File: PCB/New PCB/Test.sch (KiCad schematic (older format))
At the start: 38 parts, among them P10 CONN_2, P11 CONN_2, P12 CONN_1, P13 CONN_1, P14 CONN_1, P15 CONN_1, P16 CONN_6, P2 PROG_H, P3 CONN_2, P6 CONN_2, P7 CONN_2, P8 CONN_2, P9 CONN_2, U1 DSPIC33EP512MC806

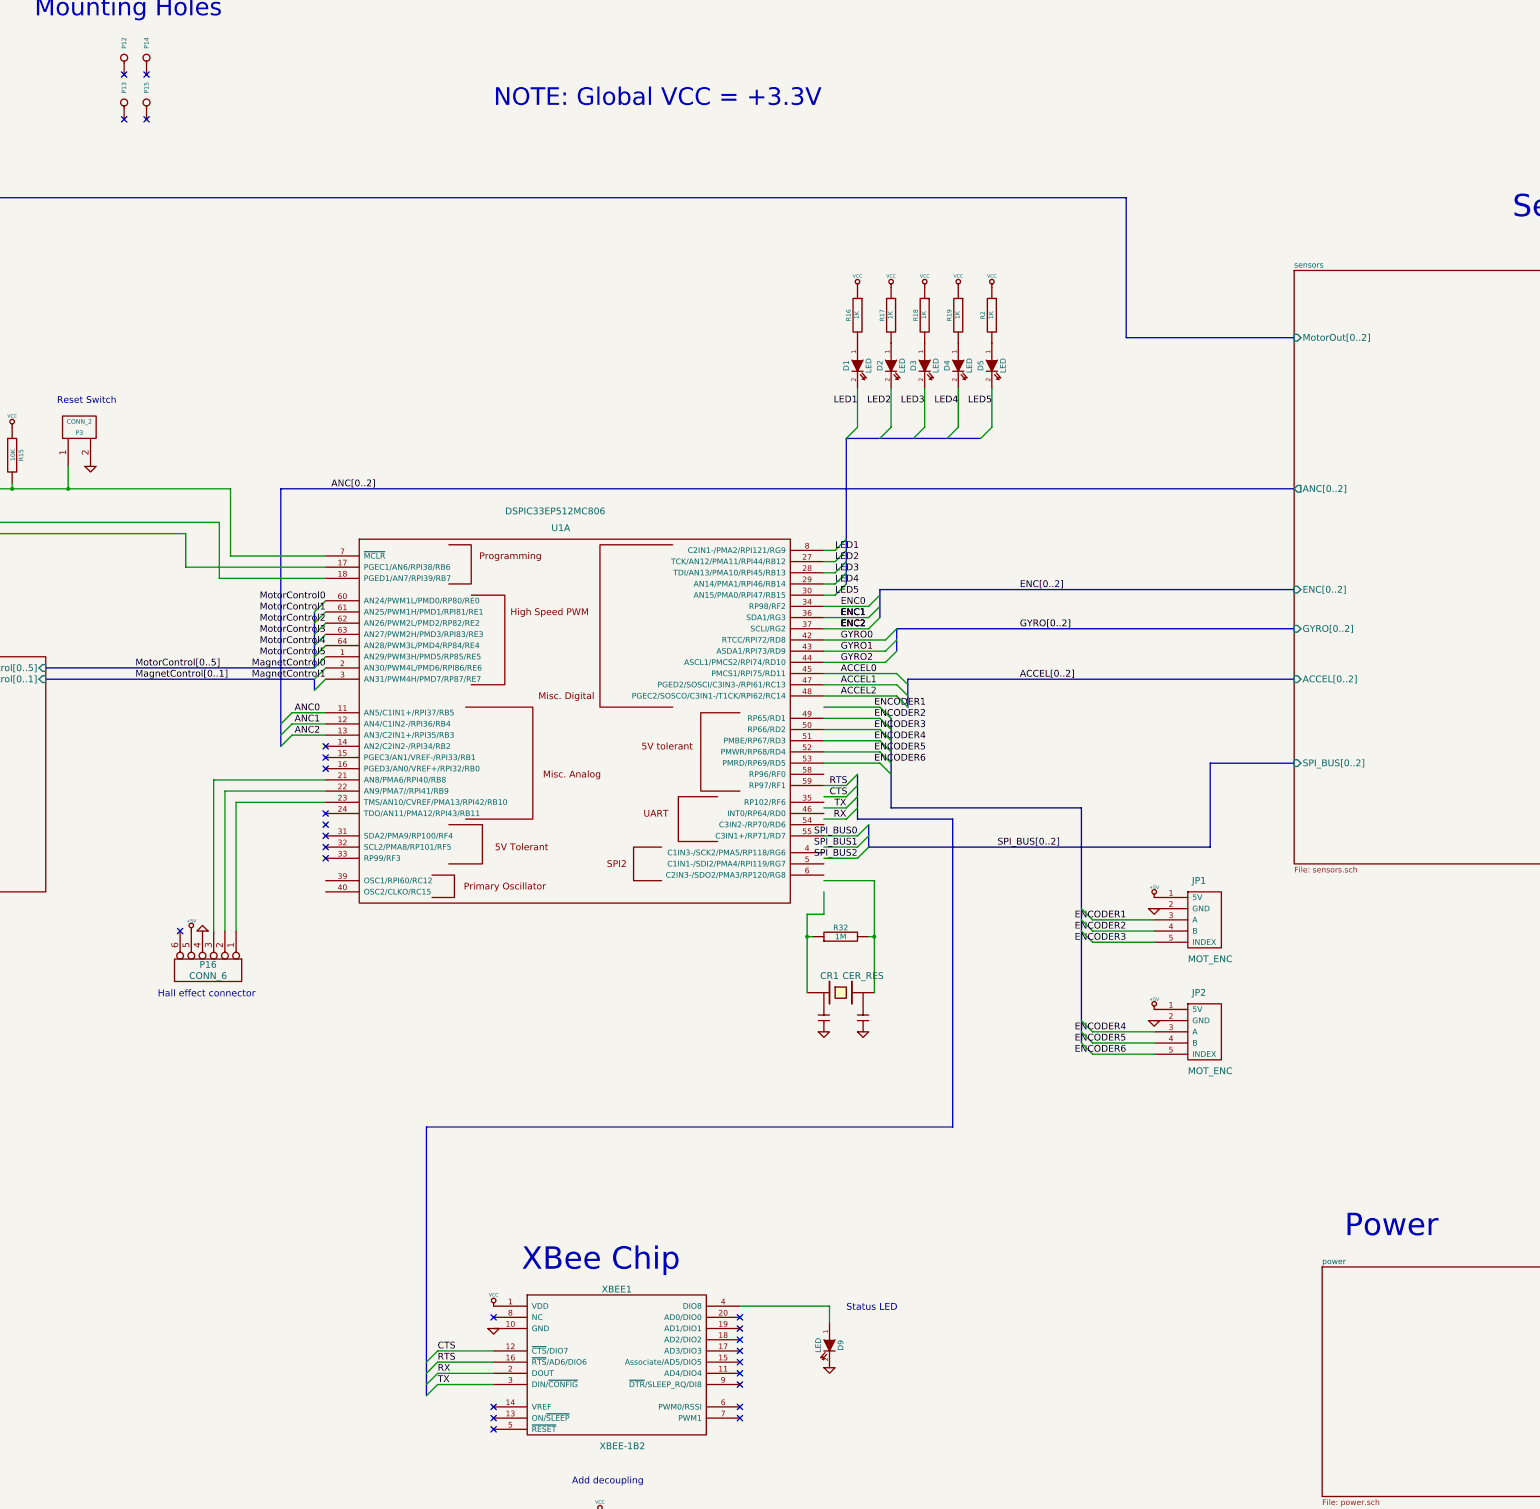
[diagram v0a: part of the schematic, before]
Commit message: order has been placed and confirmed, receipt in project folder
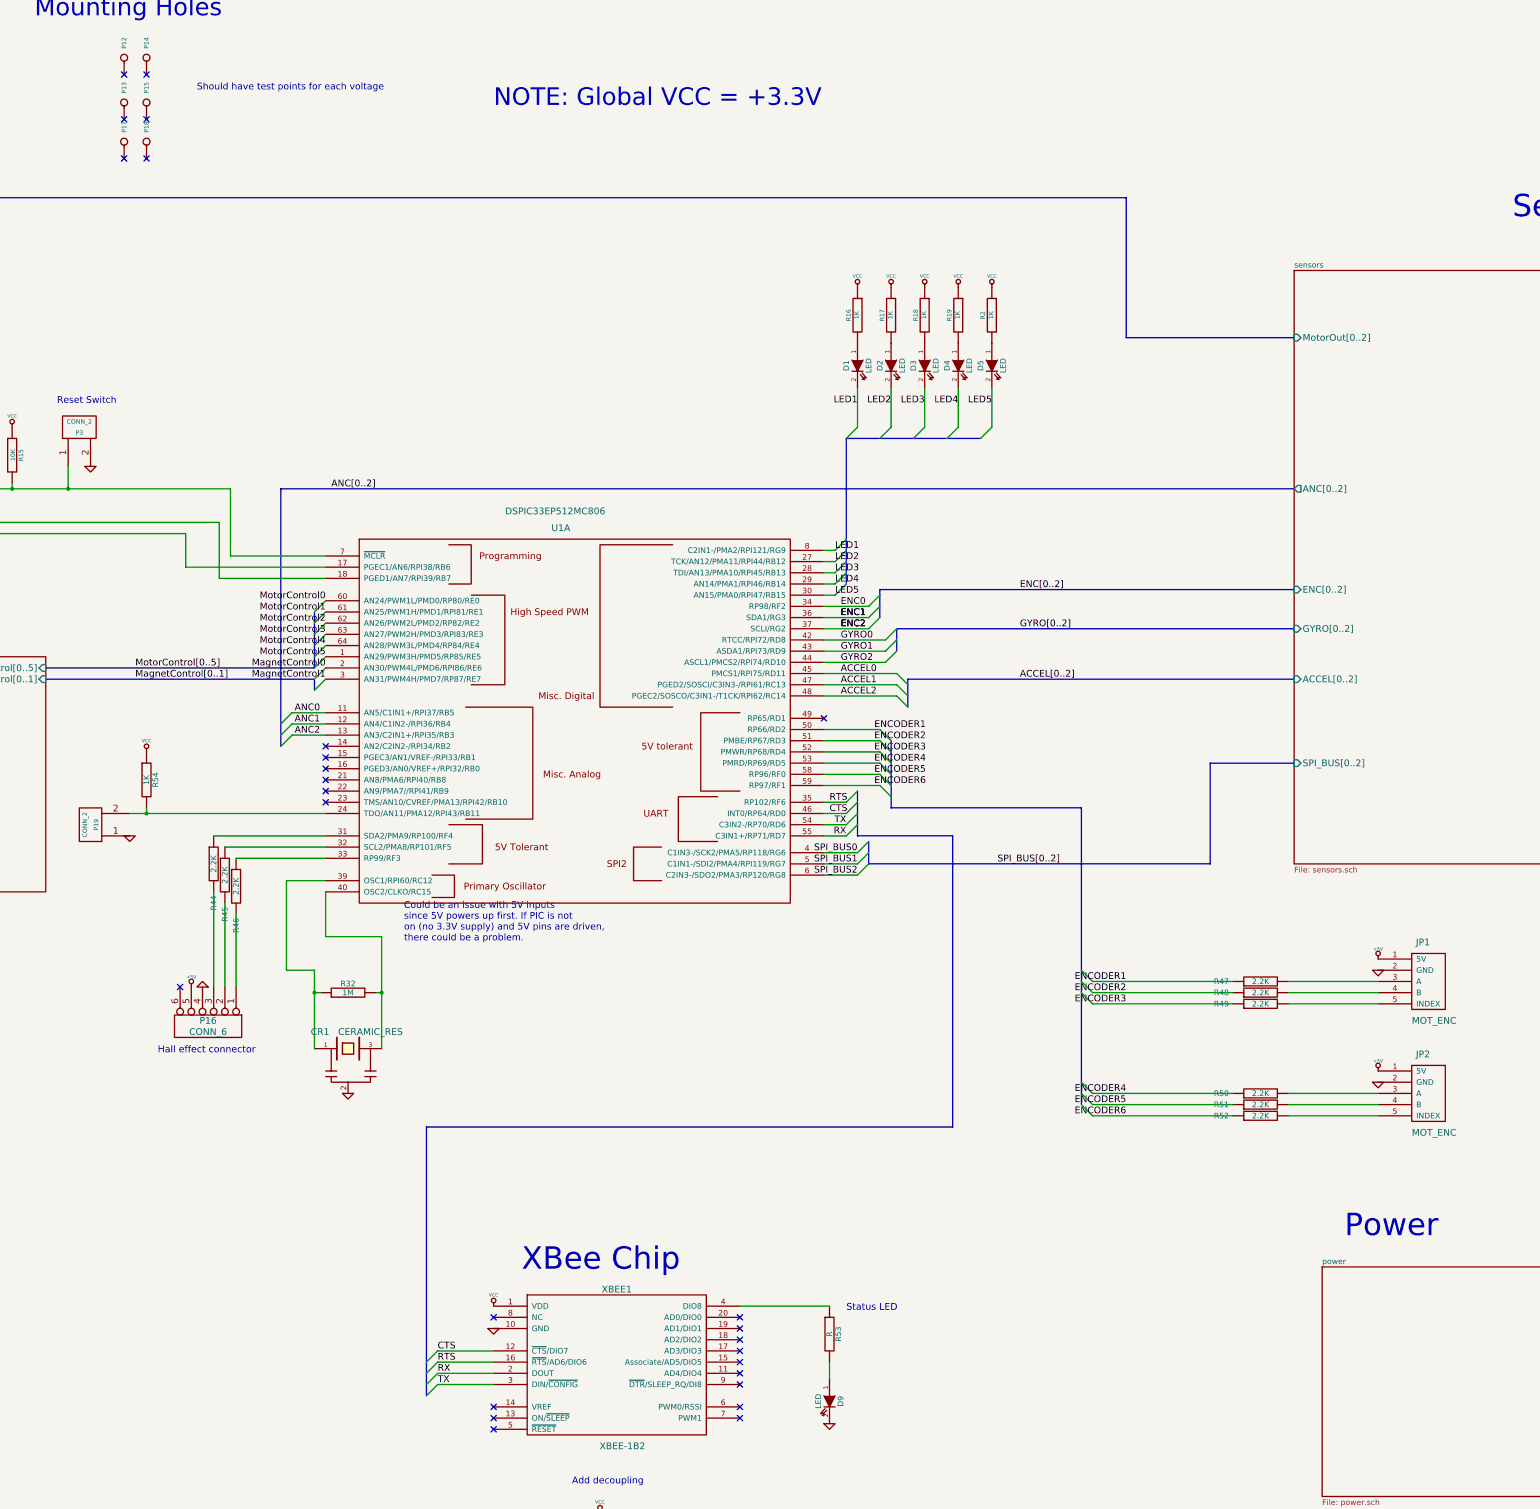
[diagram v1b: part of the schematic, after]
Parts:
- removed CR1: CER_RES, symbol CER_RES
- added CR1: CERAMIC_RES, symbol CERAMIC_RES
- added P17, P18: CONN_1, symbol CONN_1
- added P19: CONN_2, symbol CONN_2
- added R44, R45, R46, R47, R48, R49, R50, R51, R52: 2.2K, ~, symbol R
- added R53: R, ~, symbol R
- added R54: 1K, ~, symbol R
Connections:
- wire segments 77 -> 87
- no-connect marks 26 -> 27
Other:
- note added: "Could be an issue with 5V inputs\nsince 5V powers up first. If PIC is not\non (no 3.3V supply) and 5V pins are driven,\nthere could be a problem."
- note added: "Should have test points for each voltage"
- moved on the sheet: D9, JP1, JP2, P16, R32
